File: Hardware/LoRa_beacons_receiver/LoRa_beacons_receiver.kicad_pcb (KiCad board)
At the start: 2 copper layers, 65 x 50 mm, 45 parts, among them J1 Conn_Coaxial, J2 USB_C_Receptacle_USB2.0_16P, J3 I2C_Display, J4 ST-Link, J5 1PPS_out, J6 Conn_02x09_Counter_Clockwise, SW1 RST_button, SW2 BOOT_button, U1 STM32WLE5JC, U2 CP2102N-Axx-xQFN28, U3 AP2112K-3.3, U4 74LVC1G175

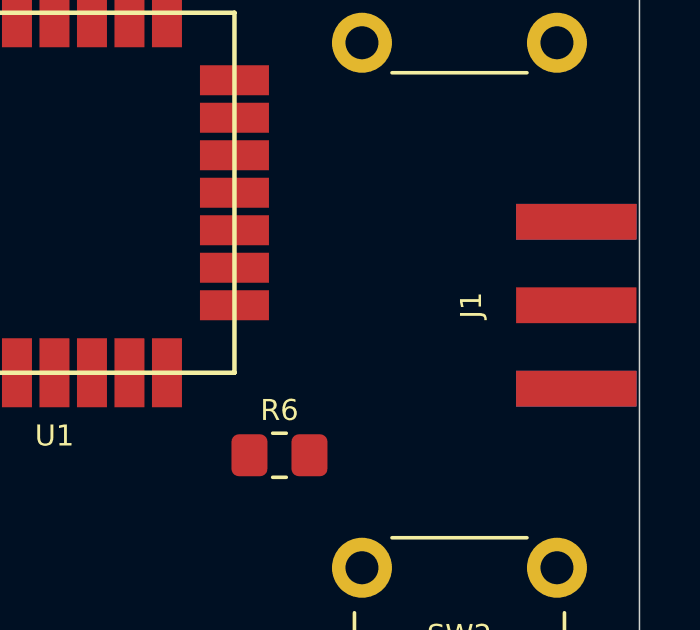
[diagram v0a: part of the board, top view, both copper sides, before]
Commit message: Clenaup
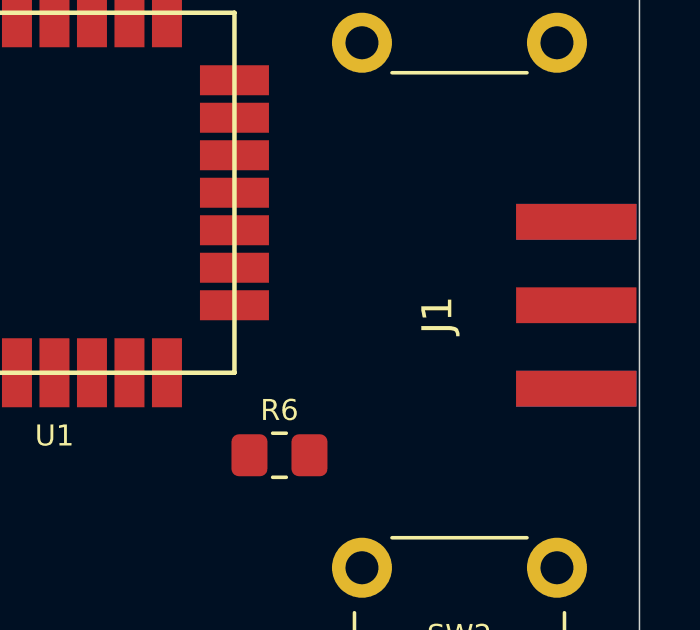
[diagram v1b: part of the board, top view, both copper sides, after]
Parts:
- J1: footprint Connector_Coaxial_g:RF2-143-T-17-50-G -> Connector_Coaxial_l:RF2-143-T-17-50-G_l
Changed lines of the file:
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@@
 		)
 		(embedded_fonts no)
-		(model "${KIPRJMOD}/symbols/STM32_module_l.pretty/STM32WLE5JC_3D.stp"
+		(model "${KIPRJMOD}/3dmodels/STM32WLE5JC_3D_l.stp"
 			(offset
 				(xyz 0 0 2.5)
 			)
 			(scale
-				(xyz 0.0385 0.0385 0.0385)
+				(xyz 0.0395 0.0395 0.0395)
 			)
 			(rotate
@@
 		)
 		(embedded_fonts no)
-		(model "${KIPRJMOD}/symbols/Diode_SMD_l.pretty/MBR130LSFT1G.stp"
+		(model "${KIPRJMOD}/3dmodels/MBR130LSFT1G_l.stp"
 			(offset
 				(xyz 0 0 0)
@@
 			)
 		)
-		(model "${KIPRJMOD}/symbols/Display_l.pretty/OLED_0_96INCH.step"
+		(model "${KIPRJMOD}/3dmodels/OLED_0_96INCH_l.step"
 			(offset
 				(xyz 0 -9.15 11.5)
@@
 		)
 	)
-	(footprint "Connector_Coaxial_g:RF2-143-T-17-50-G"
+	(footprint "Connector_Coaxial_l:RF2-143-T-17-50-G_l"
 		(layer "F.Cu")
 		(at 164.9 74 90)
 		(property "Reference" "J1"
-			(at 0 -5.5066 90)
+			(at -0.325 -6.635 90)
 			(layer "F.SilkS")
 			(effects
 				(font
-					(size 0.7 0.7)
-					(thickness 0.1)
+					(size 1 1)
+					(thickness 0.15)
 				)
 			)
@@
 		)
 		(embedded_fonts no)
-		(model "C:/Users/DELL_KM/Documents/KiCad/9.0/3dmodels/RF2-143-T-17-50-G.step"
+		(model "${KIPRJMOD}/3dmodels/RF2-143-T-17-50-G_l.step"
 			(offset
 				(xyz 0 0 0)
